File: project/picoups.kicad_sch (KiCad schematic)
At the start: 42 parts, among them J1 Conn_02x20_Odd_Even, J2 BATT, J3 VIN, J4 5V, Q1 Q_PMOS_GSD, U1 LT3652EMSE, U2 INA3221, U3 TPS61235P

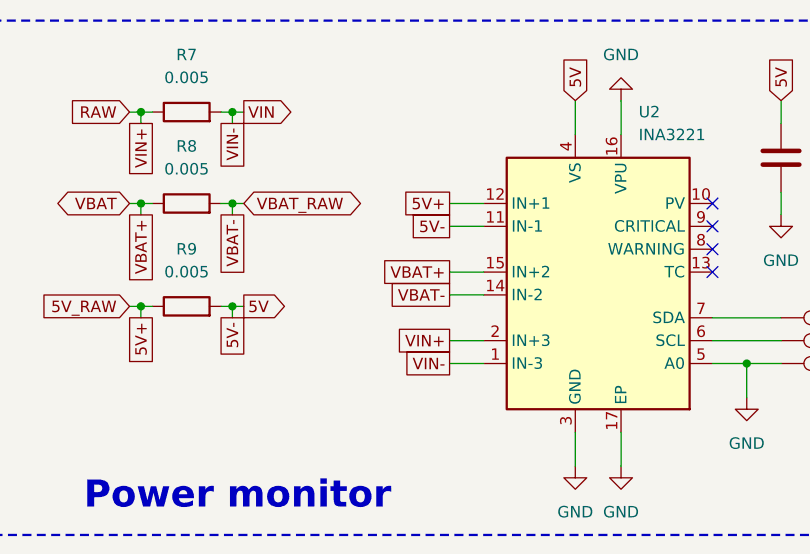
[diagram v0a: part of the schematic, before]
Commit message: Semi final layout
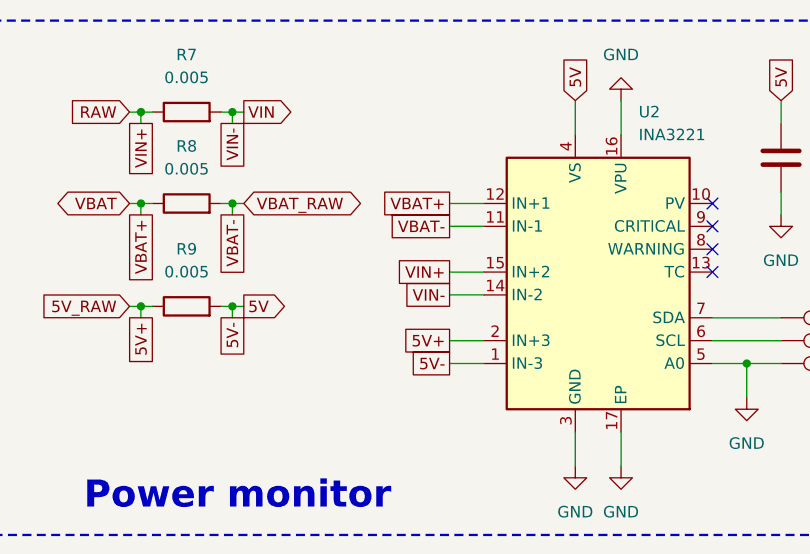
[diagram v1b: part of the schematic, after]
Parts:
- J4: footprint Connector_JST:JST_PH_B2B-PH-K_1x02_P2.00mm_Vertical -> Connector_JST:JST_PH_S2B-PH-K_1x02_P2.00mm_Horizontal
- L1: footprint Inductor_SMD:L_Wuerth_HCI-1050 -> Inductor_SMD:L_Abracon_ASPI-4030S
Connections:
- net 5V: now also U2.1 (IN-3); no longer U2.11 (IN-1)
- net 5V+: now also U2.2 (IN+3); no longer U2.12 (IN+1)
- net RAW: now also U2.15 (IN+2); no longer U2.2 (IN+3)
- net VBAT: now also U2.12 (IN+1); no longer U2.15 (IN+2)
- net VBAT-: now also U2.11 (IN-1); no longer U2.14 (IN-2)
- net VIN: now also U2.14 (IN-2); no longer U2.1 (IN-3)
